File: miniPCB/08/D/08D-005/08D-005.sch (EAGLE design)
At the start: 43 parts, among them U1 OPAMP_QUADTHD

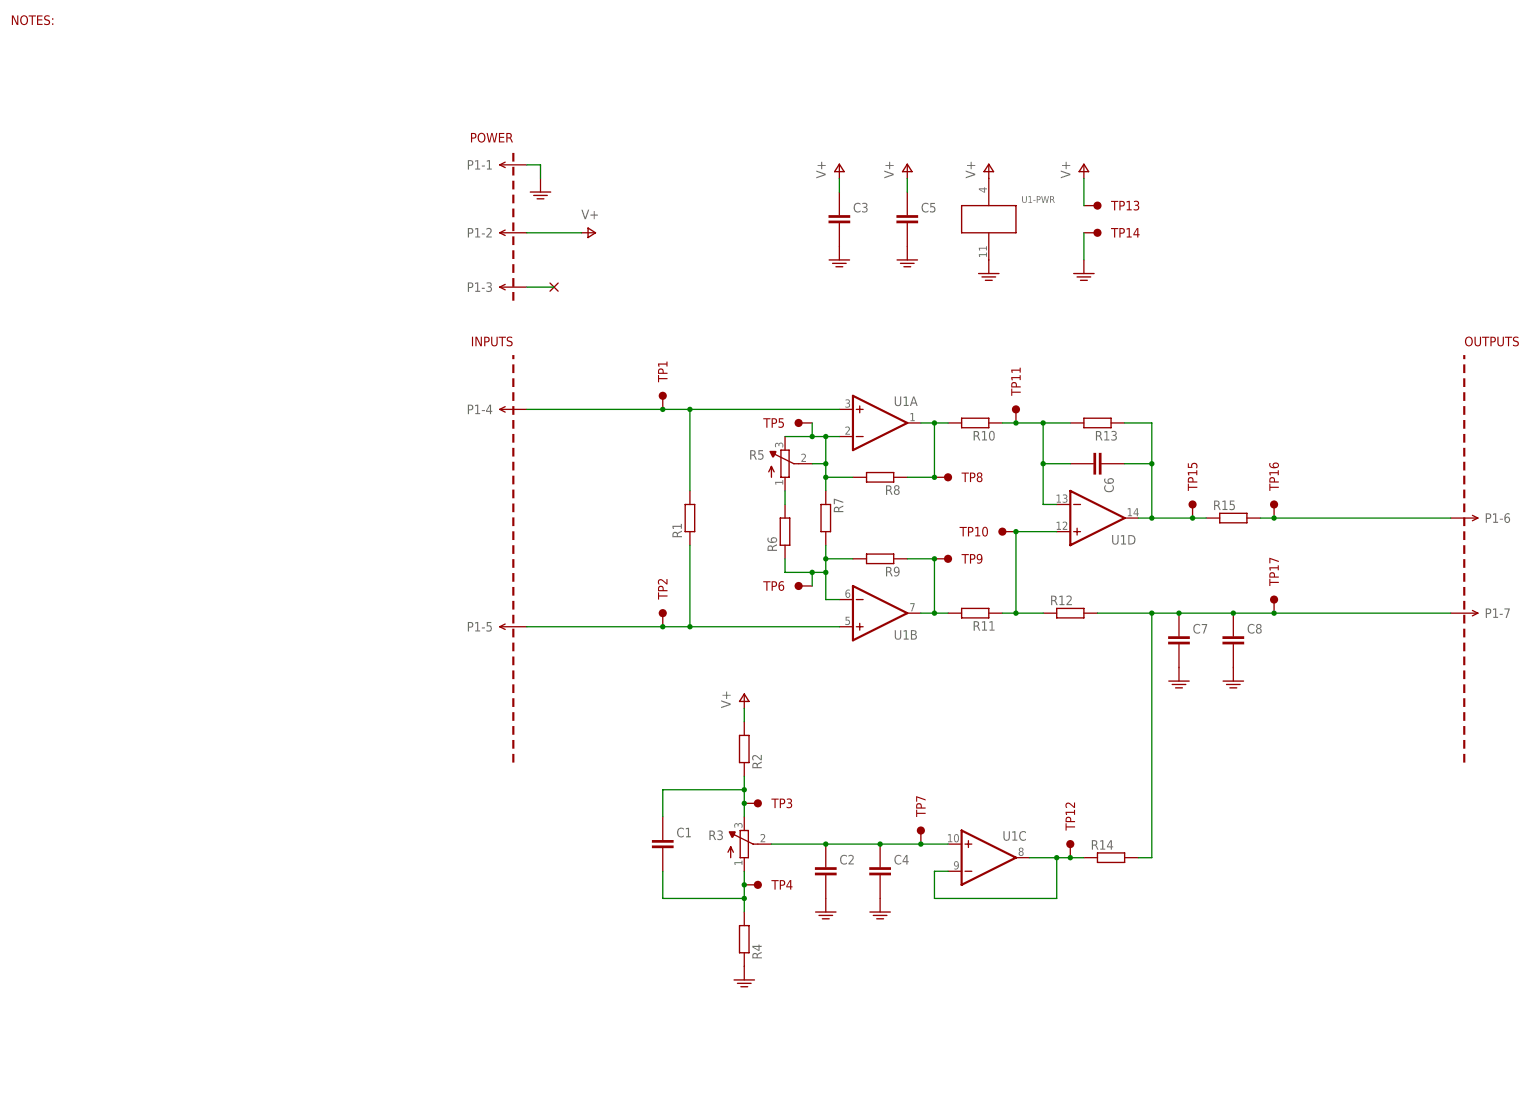
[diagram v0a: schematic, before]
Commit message: Attempting to fix my Git merge error.
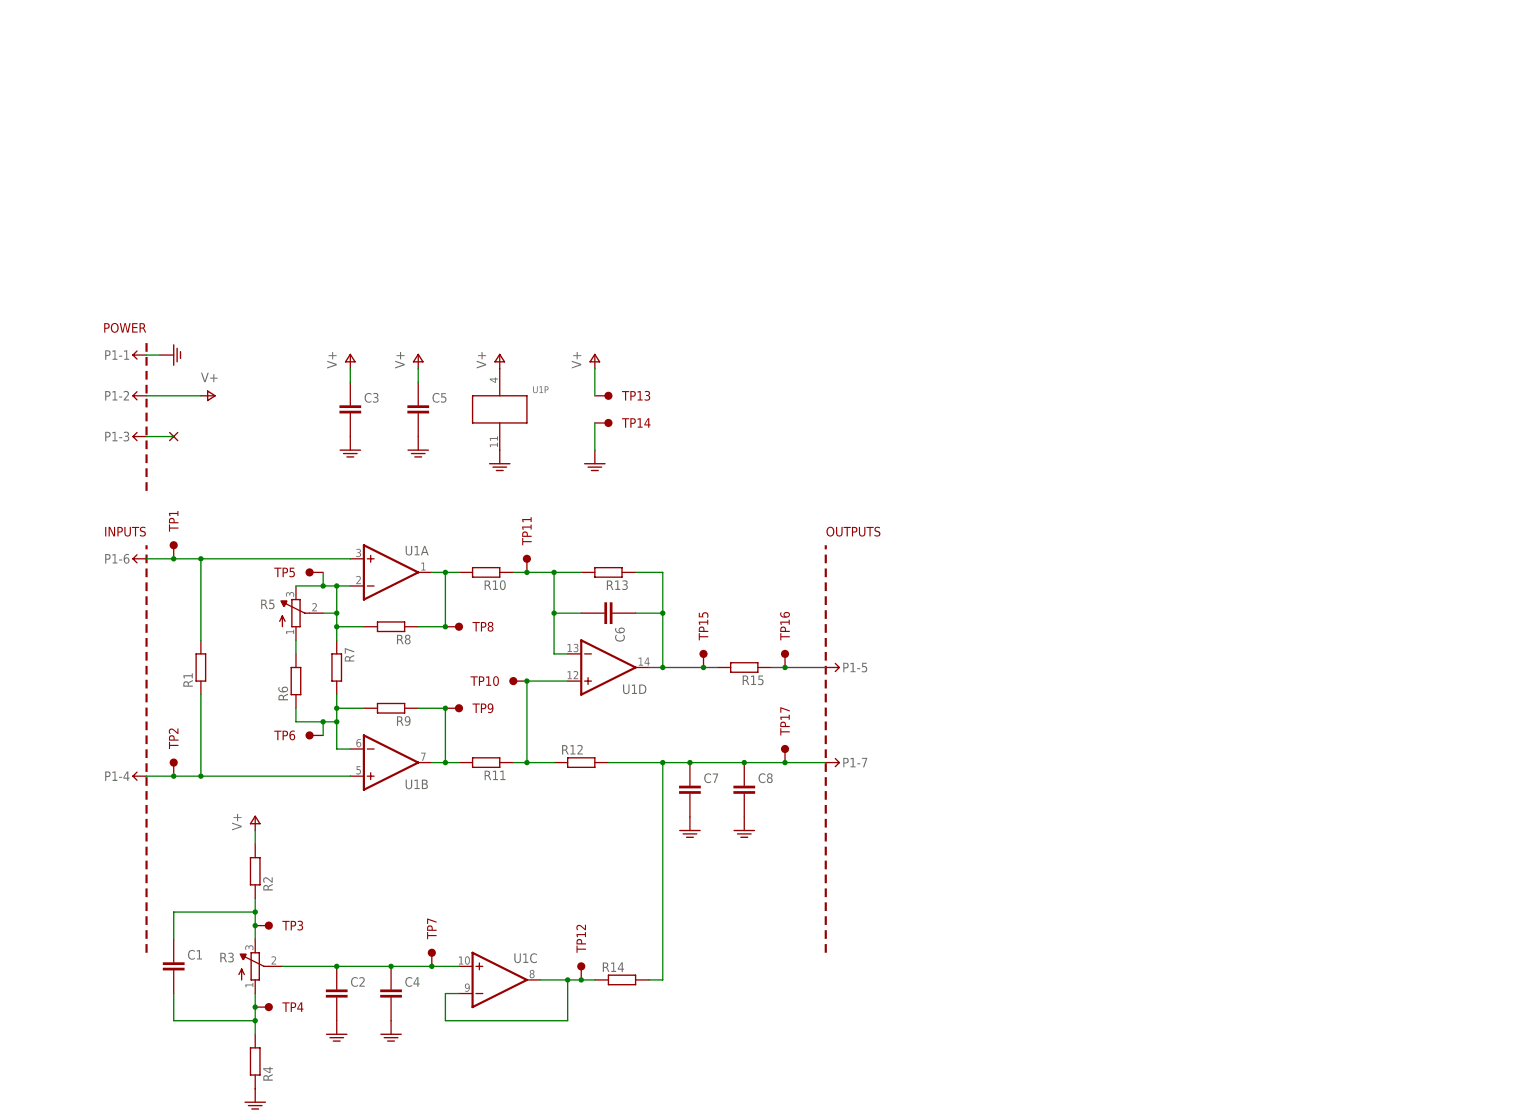
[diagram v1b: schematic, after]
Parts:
- removed P1: (no value), minipcb:MINIPCB_7P
- removed PCB1: (no value), minipcb:MINIPCB_0P50X75
- added P1-: (no value), minipcb:MINIPCB_7P50X100
- C4, C5, C8: device minipcb:CAPACITOR_10 -> minipcb:CAPACITORTHD
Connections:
- net GND: now also P1-1.1, U1P.V-; no longer P1-1.1, U1-PWR.V-
- net N$11: now also P1-5.1, R15.1; no longer P1-6.1, R15.2
- net N$2: now also P1-7.1; no longer P1-7.1
- net N$3: now also P1-4.1; no longer P1-5.1
- net N$4: now also P1-6.1; no longer P1-4.1
- net NC: now also P1-3.1; no longer P1-3.1
- net OUT: now also R15.2; no longer R15.1
- net V+: now also P1-2.1, U1P.V+; no longer P1-2.1, U1-PWR.V+
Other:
- note removed: "NOTES:"
- moved on the sheet: C1, C2, C3, C4, C5, C6, C7, C8, R1, R10, R11, R12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

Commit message: Attempting to fix my Git merge error.
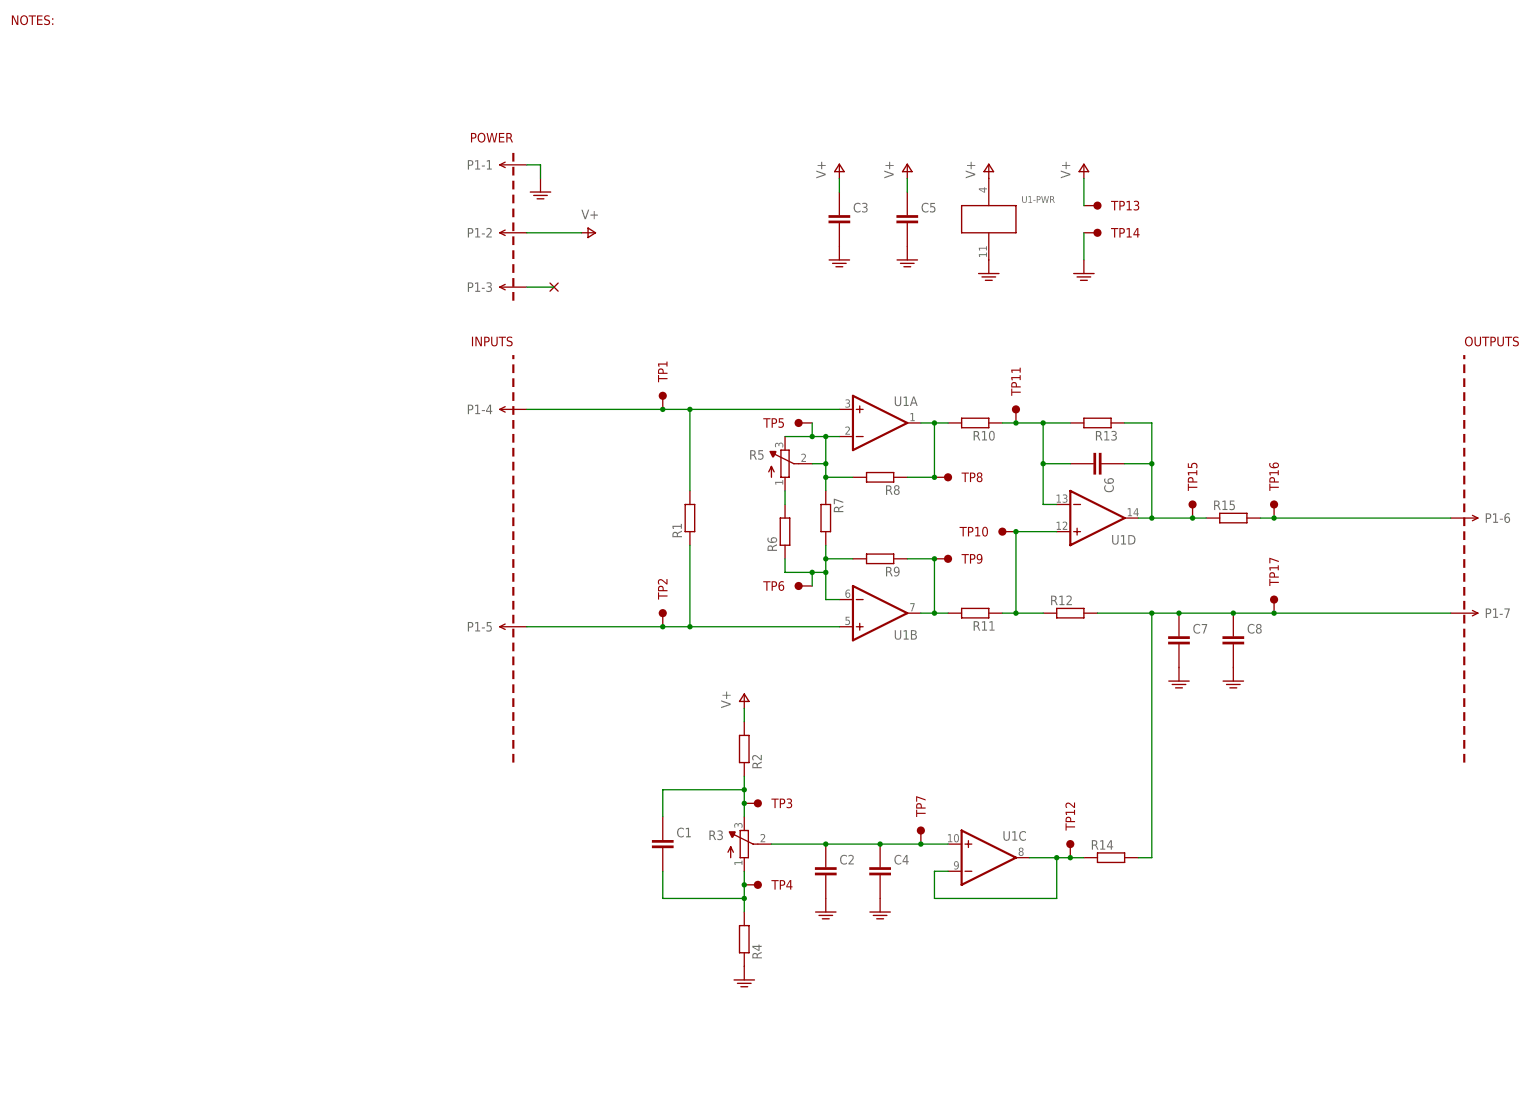
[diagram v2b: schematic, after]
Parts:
- removed P1-: (no value), minipcb:MINIPCB_7P50X100
- added P1: (no value), minipcb:MINIPCB_7P
- added PCB1: (no value), minipcb:MINIPCB_0P50X75
- C4, C5, C8: device minipcb:CAPACITORTHD -> minipcb:CAPACITOR_10
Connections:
- net GND: now also P1-1.1, U1-PWR.V-; no longer P1-1.1, U1P.V-
- net N$11: now also P1-6.1, R15.2; no longer P1-5.1, R15.1
- net N$2: now also P1-7.1; no longer P1-7.1
- net N$3: now also P1-5.1; no longer P1-4.1
- net N$4: now also P1-4.1; no longer P1-6.1
- net NC: now also P1-3.1; no longer P1-3.1
- net OUT: now also R15.1; no longer R15.2
- net V+: now also P1-2.1, U1-PWR.V+; no longer P1-2.1, U1P.V+
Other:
- note added: "NOTES:"
- moved on the sheet: C1, C2, C3, C4, C5, C6, C7, C8, R1, R10, R11, R12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
